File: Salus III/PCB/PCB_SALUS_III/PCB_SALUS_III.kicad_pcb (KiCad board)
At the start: 2 copper layers, 100 x 100 mm, 47 parts, among them J1 Conn_01x20_Pin, J2 Conn_01x20_Pin

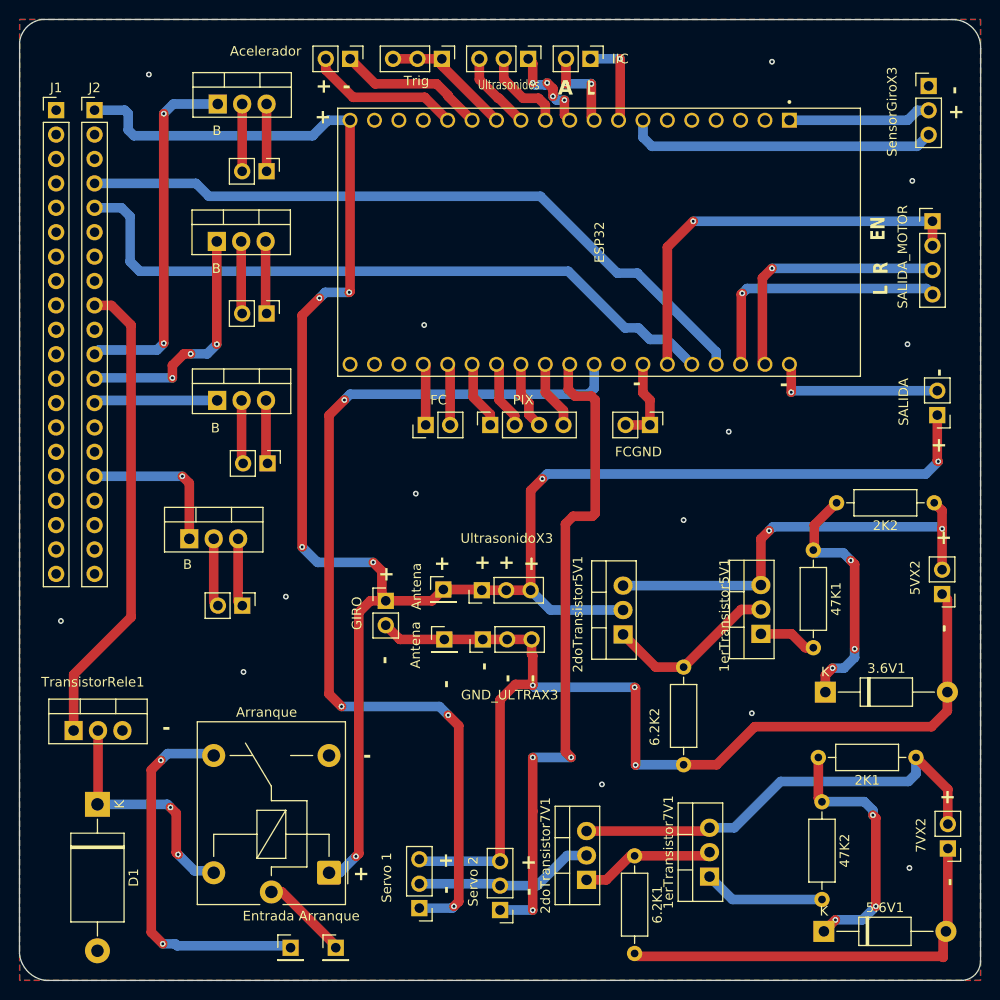
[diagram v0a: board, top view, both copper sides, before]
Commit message: Mandar a China
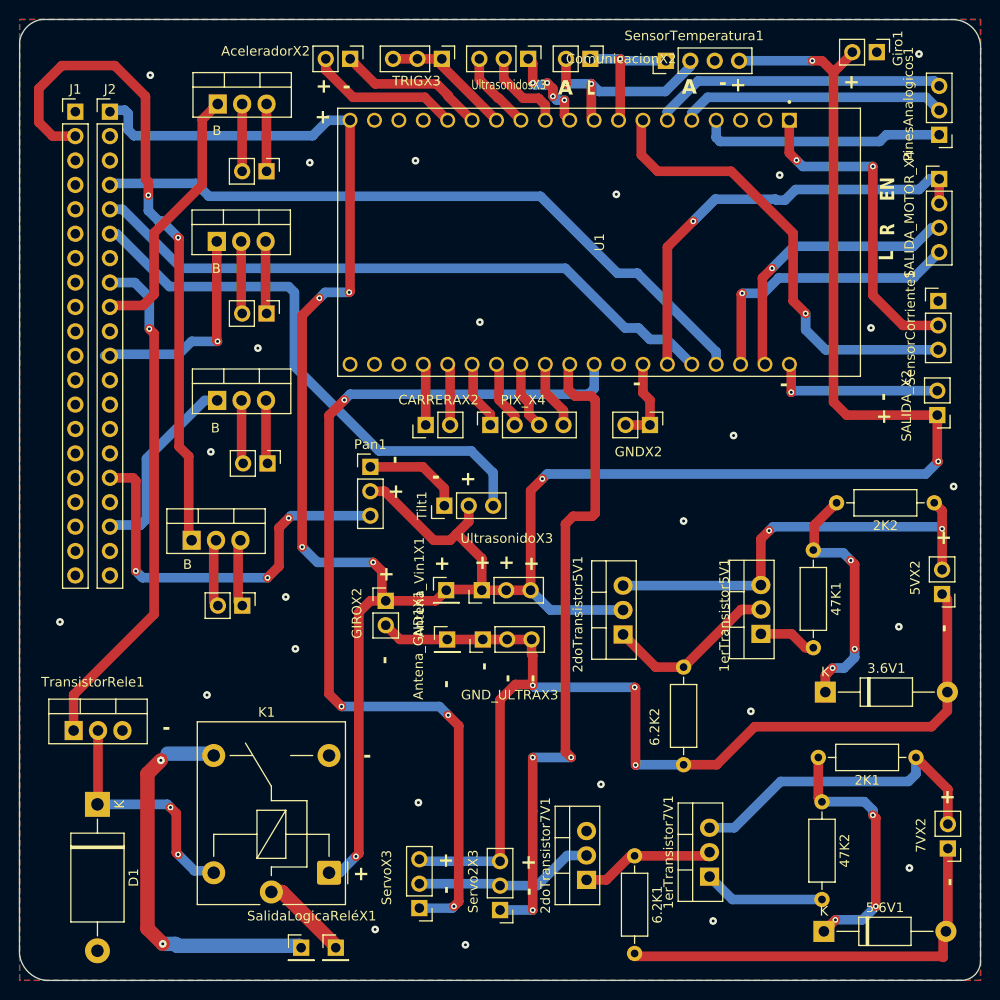
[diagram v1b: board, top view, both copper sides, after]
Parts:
- removed SensorGiroX3: Sensor de Giro, Connector_PinHeader_2.54mm:PinHeader_1x03_P2.54mm_Vertical
- added G***: LOGO, Logo:Logo, B.Cu at (318.2, 131.7)
- added Giro1: Conn_01x02_Pin, Connector_PinHeader_2.54mm:PinHeader_1x02_P2.54mm_Vertical, F.Cu at (325.4, 52.6)
- added Pan1: Conn_01x03_Pin, Connector_PinHeader_2.54mm:PinHeader_1x03_P2.54mm_Vertical, F.Cu at (272.7, 95.8)
- added PinesAnalogicos1: Conn_01x03_Pin, Connector_PinHeader_2.54mm:PinHeader_1x03_P2.54mm_Vertical, F.Cu at (331.9, 61.2)
- added SensorCorriente1: Conn_01x03_Pin, Connector_PinHeader_2.54mm:PinHeader_1x03_P2.54mm_Vertical, F.Cu at (331.8, 78.5)
- added SensorTemperatura1: Conn_01x04_Pin, Connector_PinHeader_2.54mm:PinHeader_1x04_P2.54mm_Vertical, F.Cu at (303.5, 53.5)
- added Tilt1: Conn_01x03_Pin, Connector_PinHeader_2.54mm:PinHeader_1x03_P2.54mm_Vertical, F.Cu at (280.4, 99.8)
- SalidaLogicaReléX1: renamed from Entrada Arranque
- Servo2X3: renamed from Servo 2
- ServoX3: renamed from Servo 1
- moved SALIDA_MOTOR_X4 4.46 mm to (331.9, 65.8)
- moved J1 2.01 mm to (242.0, 58.8)
- moved J2 1.61 mm to (245.6, 58.8)
- moved SalidaLogicaReléX1 1.10 mm to (265.5, 145.8)
- moved Antena_Vin1X1 0.31 mm to (280.6, 108.6)
- moved Antena_GND1X1 0.30 mm to (280.7, 113.7)
- moved TransistorLogica4 0.29 mm to (254.1, 103.4)
- renumbered Acelerador to AceleradorX2, Antena to Antena_GND1X1, Antena to Antena_Vin1X1, FC to CARRERAX2, IIC to ComunicacionX2, GIRO to GIROX2, FCGND to GNDX2, Arranque to K1, PIX to PIX_X4, SALIDA_MOTOR to SALIDA_MOTOR_X4, SALIDA to SALIDA_X2, Trig to TRIGX3, ESP32 to U1, Ultrasonidos to UltrasonidosX3
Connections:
- J1 pad 2: unconnected-(J1-Pin_2-Pad2) -> Net-(J1-Pin_2)
- J2 pad 12: Net-(J2-Pin_12) -> unconnected-(J2-Pin_12-Pad12)
- J2 pad 13: Net-(J2-Pin_13) -> unconnected-(J2-Pin_13-Pad13)
- J2 pad 18: unconnected-(J2-Pin_18-Pad18) -> Net-(J2-Pin_18)
- J2 pad 6: unconnected-(J2-Pin_6-Pad6) -> Net-(J2-Pin_6)
- J2 pad 8: unconnected-(J2-Pin_8-Pad8) -> Net-(J2-Pin_8)
- TransistorLogica1 pad 1: Net-(J2-Pin_11) -> Net-(J2-Pin_9)
- TransistorLogica2 pad 1: Net-(J2-Pin_12) -> Net-(J2-Pin_11)
- TransistorLogica3 pad 1: Net-(J2-Pin_13) -> Net-(J2-Pin_18)
- TransistorLogica4 pad 1: Net-(J2-Pin_16) -> Net-(J1-Pin_2)
- TransistorRele1 pad 1: Net-(J2-Pin_9) -> Net-(J2-Pin_8)
- U1 pad J2-4: unconnected-(U1-SENSOR_VN-PadJ2-4) -> Net-(PinesAnalogicos1-Pin_1)
- U1 pad J2-5: unconnected-(U1-IO34-PadJ2-5) -> Net-(PinesAnalogicos1-Pin_2)
- U1 pad J2-6: unconnected-(U1-IO35-PadJ2-6) -> Net-(PinesAnalogicos1-Pin_3)
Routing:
- net 5V: track 207.2 -> 286.4 mm, vias 7 -> 8
- net Net-(J1-Pin_2): track 0.00 -> 69.7 mm, vias 0 -> 2
- net Net-(J2-Pin_6): track 0.00 -> 58.1 mm
- net Net-(J2-Pin_8): track 0.00 -> 53.5 mm, vias 0 -> 1
- net Net-(PinesAnalogicos1-Pin_3): track 0.00 -> 30.7 mm
- net Net-(PinesAnalogicos1-Pin_2): track 0.00 -> 27.7 mm
- net Net-(J2-Pin_16): track 15.9 -> 41.9 mm, vias 1 -> 3
- net Net-(J2-Pin_12): track 25.7 -> 0.00 mm, vias 3 -> 0
- net Net-(PinesAnalogicos1-Pin_1): track 0.00 -> 25.5 mm
- net Net-(J2-Pin_9): track 49.3 -> 27.7 mm
- net Net-(J2-Pin_18): track 0.00 -> 20.3 mm
- net Net-(SensorCorriente1-Pin_2): track 14.9 -> 34.2 mm, vias 0 -> 2
- net Net-(SensorCorriente1-Pin_3): track 32.4 -> 48.1 mm, vias 0 -> 1
- net Net-(J2-Pin_11): track 37.6 -> 22.8 mm, vias 2 -> 1
- net Net-(J2-Pin_13): track 12.9 -> 0.00 mm
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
